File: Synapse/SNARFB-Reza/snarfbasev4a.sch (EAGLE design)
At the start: 27 parts

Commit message: computer sync
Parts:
- added BLOADER, LED8, LED9: RED, 0_jc-custom:LED0603
- added BOOT, HWB: EVQQ2, adaprog:EVQQ2
- added C10, C11, C12, C13, C14, C15, C16: 1uF, 0_jc-custom:CAP0805
- added C8, C9: 12pF, SparkFun:CAP0603-CAP
- added J1: AVR_SPI_PRG_6PTH, SparkFun:AVR_SPI_PRG_6PTH
- added LED1: red, 0_jc-custom:LED0603
- added LED10: GREEN, 0_jc-custom:LED0603
- added LED2: blue, 0_jc-custom:LED0603
- added LED3: orange, 0_jc-custom:LED0603
- added LED4: green, 0_jc-custom:LED0603
- added NX5032GA: 8MHz, adafruit:XTALNX5032
- added R10, R16, R8, R9: 220, SparkFun-Resistors:RESISTOR0805-RES
- added R11, R12, R14, R15: 1K, SparkFun-Resistors:RESISTOR0805-RES
- added R13: 10K, SparkFun-Resistors:RESISTOR0805-RES
- added R6, R7: 22, 0_jc-custom:RESISTOR0603-RES
- added SJ10: HWB, SparkFun:SOLDERJUMPERNO
- added SJ8: (no value), SparkFun:SOLDERJUMPER_2WAYPASTE2&3
- added SJ9: SOLDERJUMPERNO, SparkFun:SOLDERJUMPERNO
- added U$7: ATMEGA32U4-AU, adafruit:ATMEGA32U4-AU
- added VREG: MCP1802, 0_jc-custom:MCP1802
- added X1: USBSMD, 0_jc-custom:USBH2959CT-ND
- LM75A: device 0_jc-custom:LM75AJC-TEST -> 0_jc-custom-eagle6:LM75AJC-TEST
- R1, R2: device SparkFun:RESISTOR -> SparkFun-Resistors:RESISTOR0805-RES
- RXTX: value SERIAL_CROSSOVER -> SERIAL_CROSSOVERNORMAL; device 0_jc-custom:SERIAL_CROSSOVER -> 0_jc-custom-eagle6:SERIAL_CROSSOVERNORMAL
- VIN: value (none) -> M023.5MM; device SparkFun:M02PTH -> SparkFun-Connectors:M023.5MM
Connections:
- removed net GPIO3: RFE.GPIO3_RX_UART0, RFE.P$29, RFE.P$5
- removed net GPIO4: RFE.GPIO4_TX_UART0, RFE.P$30, RFE.P$6
- new net AREF-7: U$7.AREF
- new net HWB: HWB.P, HWB.P1, R13.1, SJ10.1, U$7.PE2(HWB)
- new net MISO: J1.1, U$7.PB3(PDO/MISO)
- new net MOSI: J1.4, U$7.PB2(PDI/MISO)
- new net MVOUT: C12.1, R11.2, SJ9.1, VREG.VOUT
- new net N$1: LED2.A, R9.2
- new net N$10: BLOADER.C, R12.1
- new net N$13: LED4.A, R16.2
- new net N$2: LED3.A, R10.2
- new net N$4: C10.2, U$7.UCAP
- new net N$5: LED9.C, R15.1
- new net N$6: LED1.A, R8.2
- new net N$8: LED10.A, R11.1
- new net N$9: LED8.C, R14.1
- new net PB4-GRN-L4: R16.1, U$7.PB4(ADC11)
- new net PB5-ORANGE-L3: R10.1, U$7.PB5(OC1A/OC4B/ADC12)
- new net PB6-BLUE-L2: R9.1, U$7.PB6(OC1B/OC4B/ADC13)
- new net PB7-RED-L1: R8.1, U$7.PB7(OC0A/OC1C/RTS)
- new net PC6-LED8: LED8.A, U$7.PC6(OC1A)
- new net PC7-LED9: LED9.A, U$7.PC7(ICP3/CLK0/OC4A)
- new net PD4: U$7.PD4(ICP1/ADC8)
- new net PD5: U$7.PD5(XCK/CTS)
- new net PD6: U$7.PD6(T1/OC4D/ADC9)
- new net PD7: U$7.PD7(OC4D/ADC10/T0)
- new net PE6-LED7-BOOTLOADER: BLOADER.A, U$7.PE6
- new net PF0-2: U$7.PF0(ADC0)
- new net PF1-3: U$7.PF1(ADC1)
- new net PF4-4: U$7.PF4(ADC4/TCK)
- new net PF5-5: U$7.PF5(ADC5/TMS)
- new net PF6-6: U$7.PF6(ADC6/TDO)
- new net PF7-7: U$7.PF7(ADC7(TDI)
- new net RST: BOOT.P, BOOT.P1, J1.5, U$7./RESET
- new net RX1: RFE.GPIO4_TX_UART0, RFE.P$30, RFE.P$6, U$7.PD3(INT3/TXD1)
- new net SCK: J1.3, U$7.PB1(SCK)
- new net SD_CS: U$7.PB0(SS)
- new net TX1: RFE.GPIO3_RX_UART0, RFE.P$29, RFE.P$5, U$7.PD2(INT2/RXD1)
- new net UD+: R6.2, U$7.D+
- new net UD-: R7.2, U$7.D-
- new net UDM: R7.1, X1.D-
- new net UDP: R6.1, X1.D+
- new net UVCC: SJ8.2, U$7.UVCC
- new net VBUS: C11.1, SJ8.1, U$7.VBUS, VREG.SHDN, VREG.VIN, X1.VBUS
- new net XTAL1: C9.2, NX5032GA.P$2, U$7.XTAL1
- new net XTAL2: C8.2, NX5032GA.P$1, U$7.XTAL2
- net GND: now also BOOT.S, BOOT.S1, C10.1, C11.2, C12.2, C13.2, C14.2, C15.2, C16.2, C8.1, C9.1, HWB.S, HWB.S1, J1.6, LED1.C, LED10.C, LED2.C, LED3.C, LED4.C, R12.2, R14.2, R15.2, SJ10.2, U$7.GND, U$7.GND1, U$7.GND2, U$7.GND3, U$7.UGND, VREG.GND, X1.GND
- net GPIO7: now also RXTX.RXD; no longer RXTX.4
- net GPIO8: now also RXTX.TXD; no longer RXTX.1
- net RXI: now also RXTX.RXF; no longer RXTX.3
- net SCL: now also U$7.PD0(INT0/OC0B)
- net SDA: now also U$7.PD1(INT1/SDA)
- net TXO: now also RXTX.TXF; no longer RXTX.2
- net VCC3: now also C13.1, C14.1, C15.1, C16.1, J1.2, R13.2, SJ8.3, SJ9.2, U$7.AVCC, U$7.AVCC1, U$7.VCC, U$7.VCC1
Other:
- note added: "15-14"
- note added: "23-24"
- note added: "35-34"
- note added: "43-44"
- note added: "ISP, Reset, and HWB Button"
- note added: "OR System Power"
- note added: "Opto-Isolate inputs Provide 4-8 outputs"
- note added: "Shows USB Power"
- note added: "Used by LUFA Status"
- note added: "When SJ5 is connected"
- note added: "and main program"
- note added: "for states or status"
- moved on the sheet: 24LC256, C1, C2, C3, C4, C5, C7, FTDI, LM75A, R1, R2, R3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

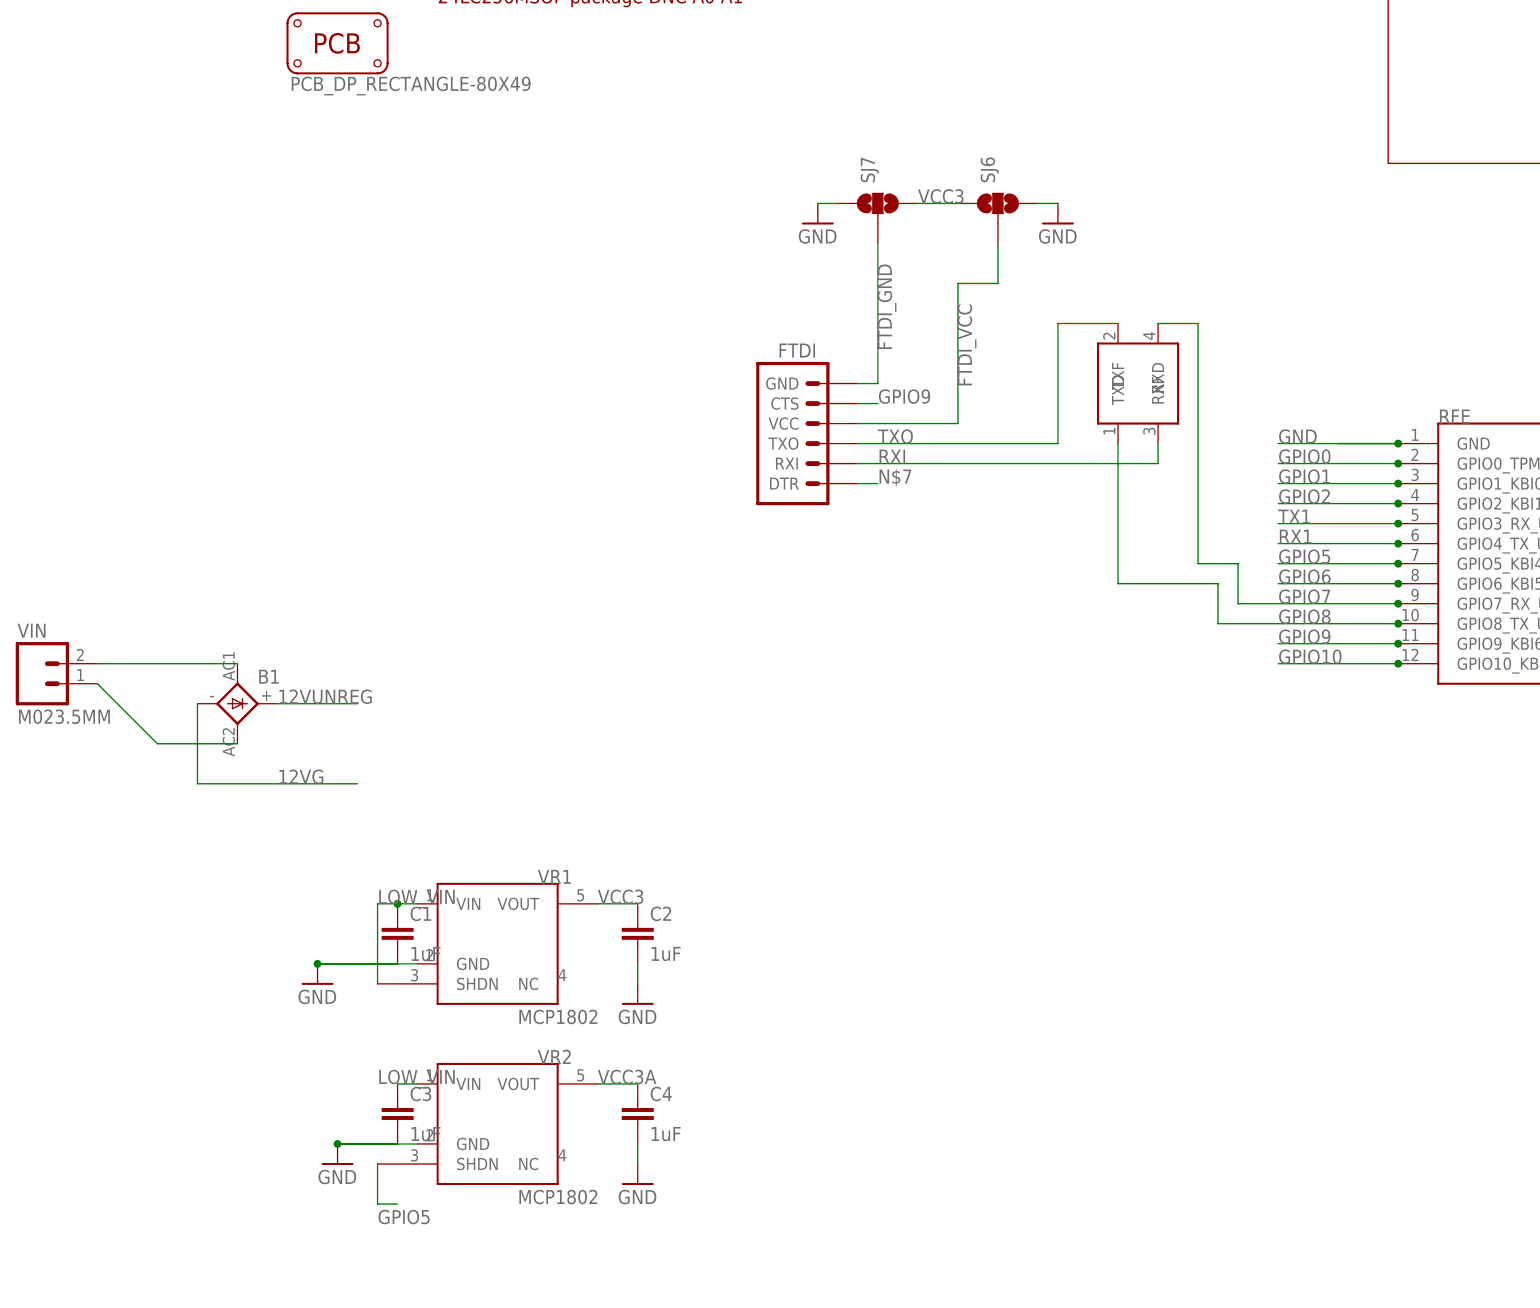
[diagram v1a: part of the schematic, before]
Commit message: place holder
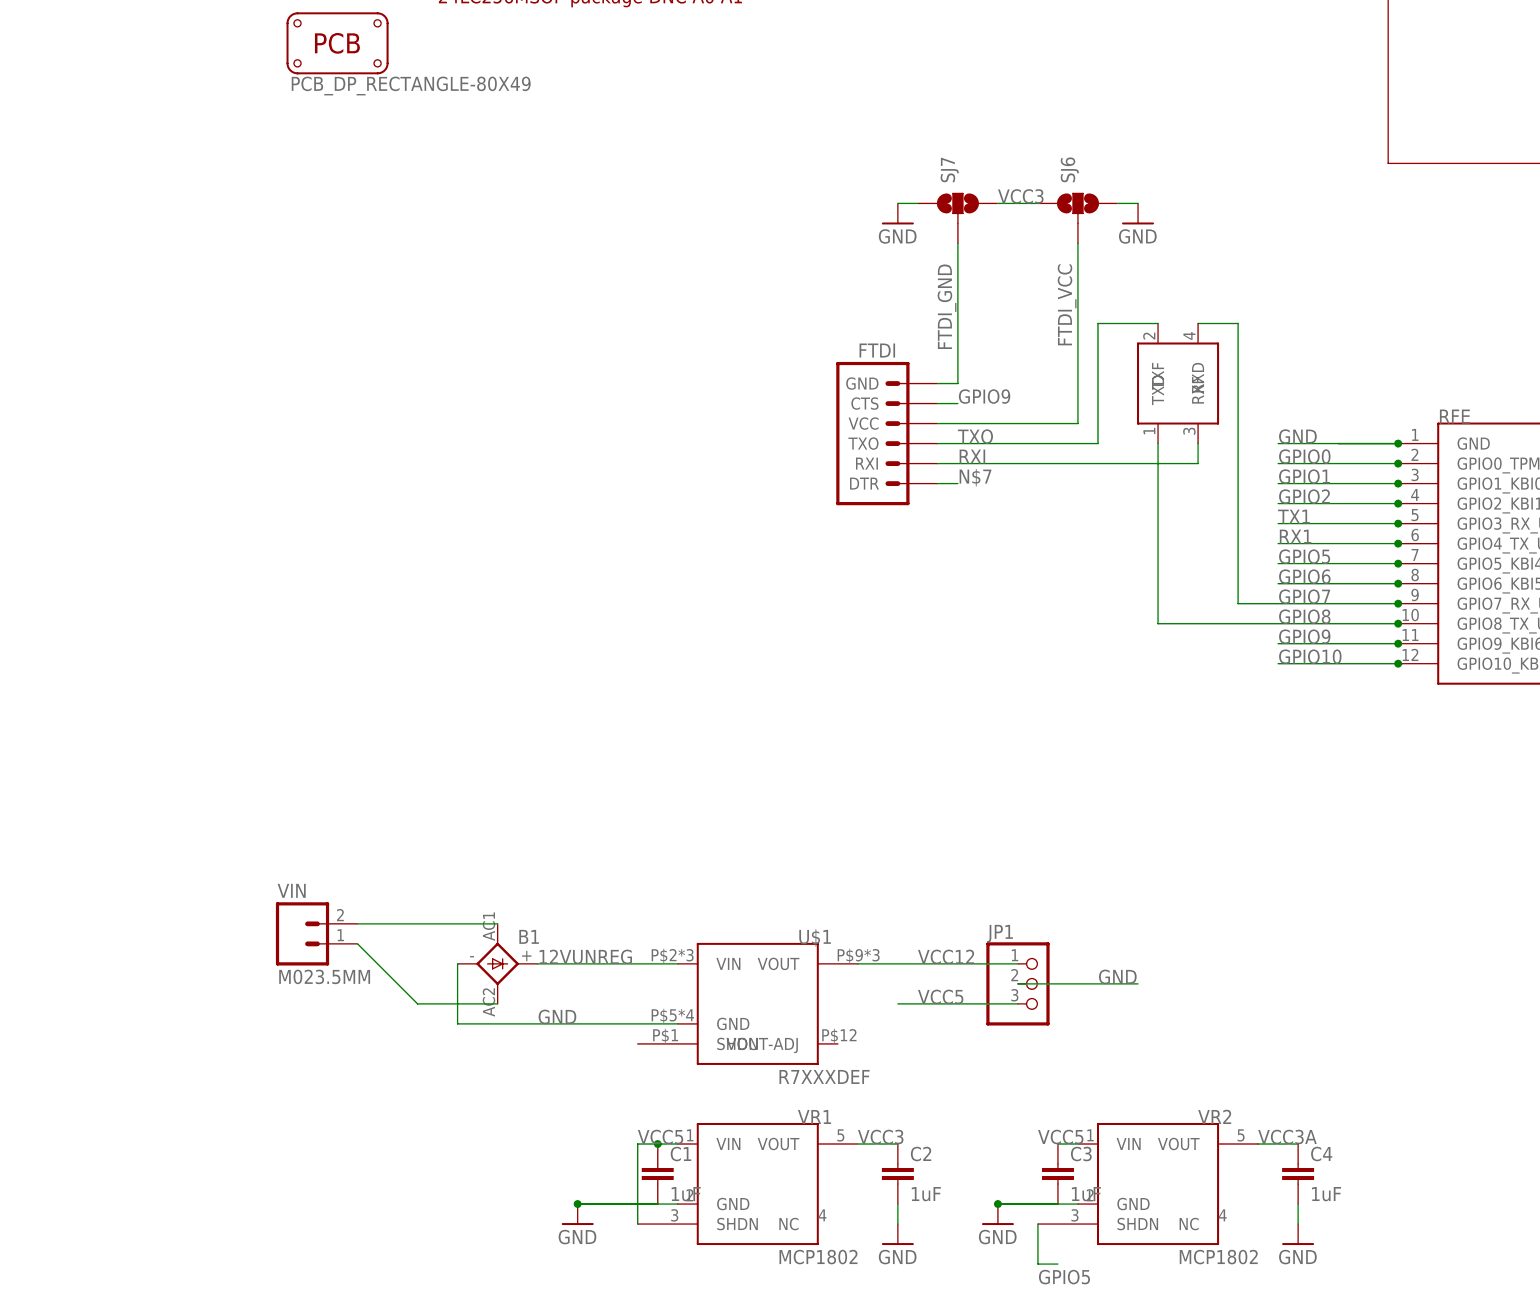
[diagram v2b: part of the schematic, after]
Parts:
- added JP1: (no value), adafruit:PINHD-1X3CB
- added U$1: R7XXXDEF, 0_jc-custom-eagle6:R7XXXDEF
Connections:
- removed net 12VG: B1.-
- removed net LOW_VIN: C1.1, C3.1, VR1.SHDN, VR1.VIN, VR2.VIN
- new net VCC12: JP1.1, U$1.VOUT
- new net VCC5: C1.1, C3.1, JP1.3, VR1.SHDN, VR1.VIN, VR2.VIN
- net 12VUNREG: now also U$1.VIN
- net GND: now also B1.-, JP1.2, U$1.GND
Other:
- moved on the sheet: B1, C1, C2, C3, C4, FTDI, SJ6, SJ7, VIN, VR1, VR2
